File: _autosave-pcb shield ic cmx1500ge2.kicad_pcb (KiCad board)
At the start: 2 copper layers, 67.9 x 53.3 mm, 52 parts, among them J1 SMA, J2 U.FL, J3 Conn_01x01_Male, J4 Conn_01x01_Male, P1 Power, P2 Analog, P3 Digital, P4 Digital, P5 HEADER2x4, P6 HEADER-1X6, P7 Communication, Q1 BSS138, Q2 BSS138, Q3 BSS138, U1 CXM1500GE, U2 TXS0108EPW, U3 LM1117-Adj, U4 ADS1115

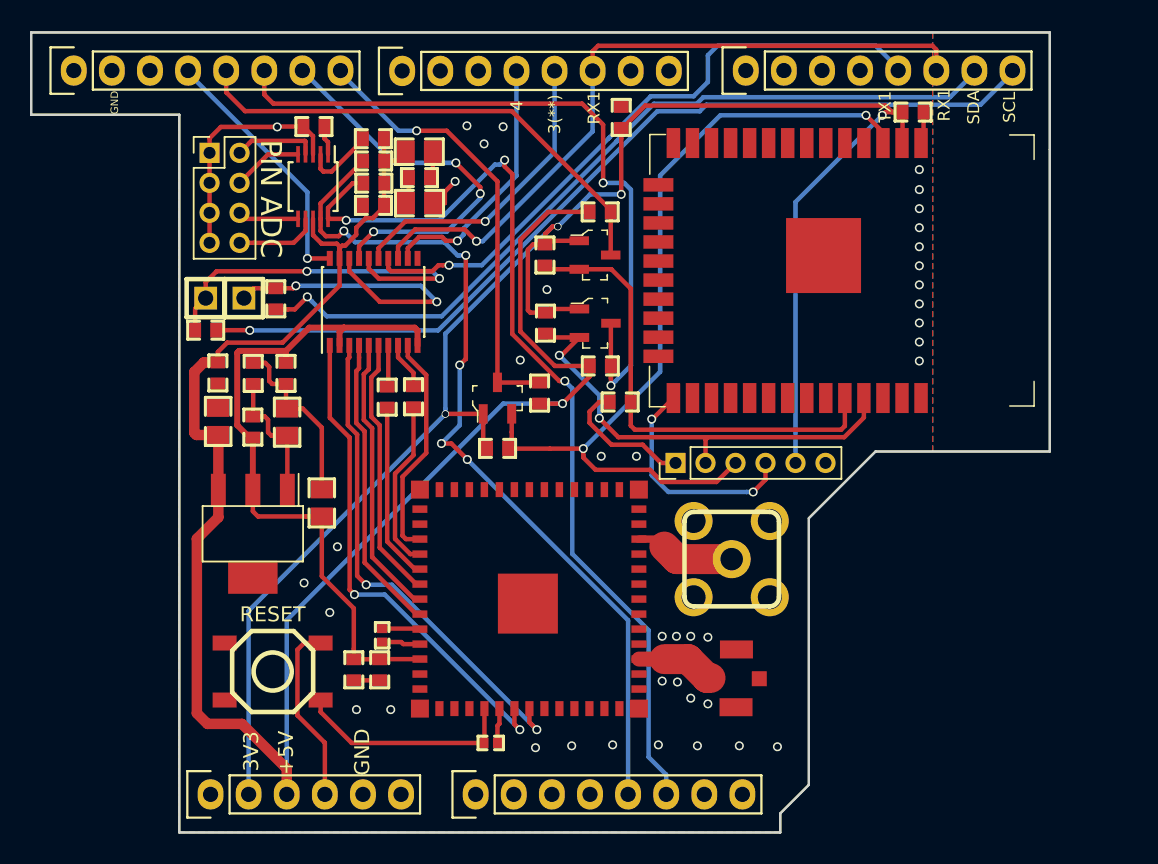
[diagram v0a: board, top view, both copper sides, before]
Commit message: initial Commit
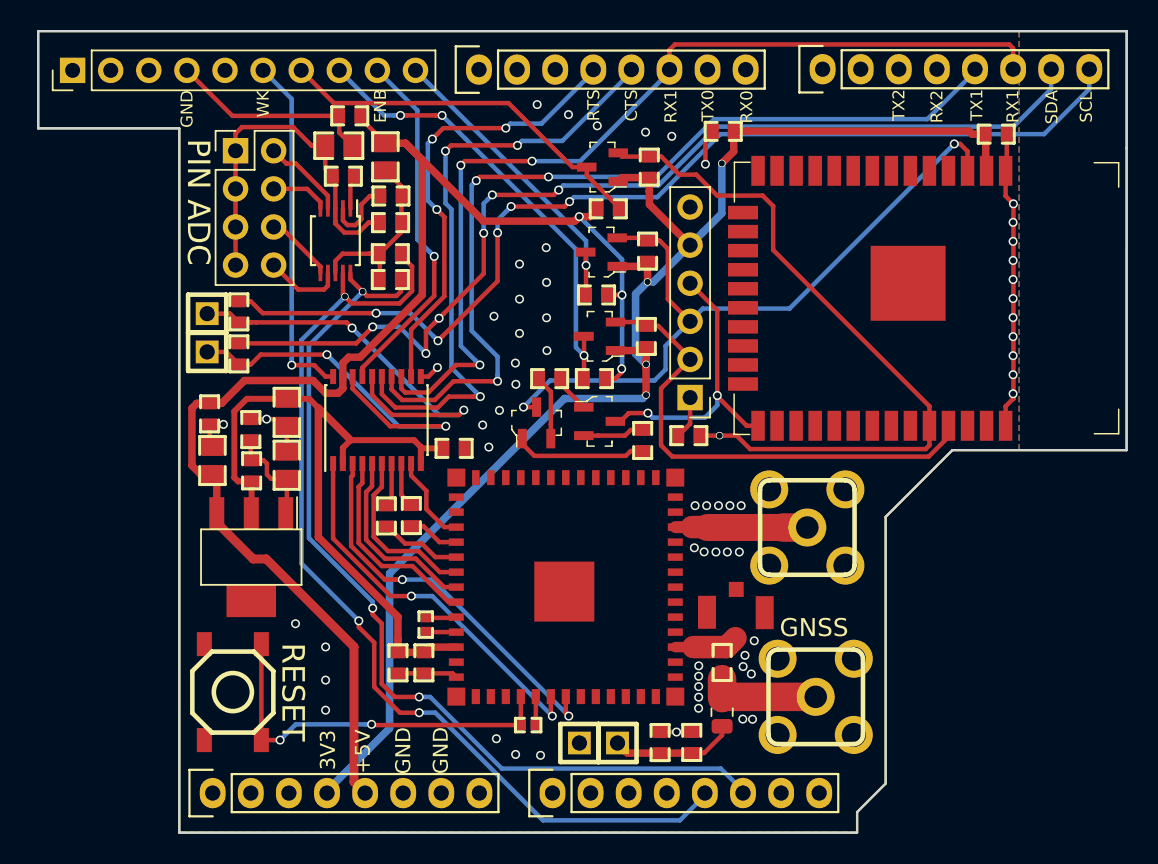
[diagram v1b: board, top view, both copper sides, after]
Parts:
- removed P3: Digital, Socket_Arduino_Uno:Socket_Strip_Arduino_1x08
- added C12: 10uF, Capasitor:C_Ceramic_SMD_0603, F.Cu at (145.2, 120.4)
- added C13: 1uF, Capasitor:C_Ceramic_SMD_0603, F.Cu at (143.1, 120.4)
- added C14: 0.1u, Capasitor:C_Ceramic_SMD_0603, F.Cu at (147.2, 115.0)
- added J5: SMA, Connectors_SMA:SMA_Male_Angled_TH, F.Cu at (153.4, 117.3)
- added J6: GND, Headers:Pin_Header_1x01_Male_10mil_Straight_TH, F.Cu at (137.7, 120.4)
- added J7: VCC, Headers:Pin_Header_1x01_Male_10mil_Straight_TH, F.Cu at (140.2, 120.4)
- added J8: Conn_01x10, Connector_PinHeader_2.54mm:PinHeader_1x10_P2.54mm_Vertical, F.Cu at (103.9, 75.6)
- added L1: 35nH, Inductor:L_0805_2012Metric, F.Cu at (147.2, 118.3)
- added Q4: S8050, digikey-footprints:SOT-23-3, F.Cu at (134.8, 99.1)
- added Q5: S8050, digikey-footprints:SOT-23-3, F.Cu at (139.0, 99.0)
- added R20: 10K, resistor:R_Chip_SMD_0603, F.Cu at (135.7, 96.1)
- added R21: 10K, resistor:R_Chip_SMD_0603, F.Cu at (141.9, 100.2)
- C5: value 10uf -> 100uf
- P1: value Power -> Analog; footprint Socket_Arduino_Uno:Socket_Strip_Arduino_1x06 -> Socket_Arduino_Uno:Socket_Strip_Arduino_1x08
- P5: footprint Connector_PinHeader_2.00mm:PinHeader_2x04_P2.00mm_Vertical -> Connector_PinHeader_2.54mm:PinHeader_2x04_P2.54mm_Vertical
- P6: footprint Connector_PinHeader_2.00mm:PinHeader_1x06_P2.00mm_Vertical -> Connector_PinHeader_2.54mm:PinHeader_1x06_P2.54mm_Vertical
- moved R10 16.5 mm to (142.2, 87.6), turned to 90 degrees
- moved C2 12.3 mm to (129.3, 100.8), turned to 180 degrees
- moved Q2 12.0 mm to (139.1, 87.7), turned to 180 degrees
- moved R9 9.09 mm to (142.3, 82.0), turned to 90 degrees
- moved R5 7.92 mm to (126.5, 105.2)
- moved R6 7.92 mm to (124.8, 105.3)
- moved U2 7.88 mm to (124.2, 98.9)
- moved R13 7.57 mm to (138.8, 90.5), turned to 0 degrees
- moved C11 6.86 mm to (147.3, 79.6), turned to 180 degrees
- moved R12 6.78 mm to (142.1, 93.3), turned to 270 degrees
- moved FB2 6.60 mm to (121.6, 80.6), turned to 180 degrees
- moved R17 6.52 mm to (125.1, 89.5), turned to 180 degrees
- moved C1 6.47 mm to (118.2, 98.4), turned to 270 degrees
- moved R18 6.28 mm to (125.1, 87.8), turned to 180 degrees
- moved C7 6.21 mm to (122.4, 78.6)
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- renumbered RESET to PB1
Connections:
- net Net-(P7-Pad3) renamed /16(Tx2)
- net Net-(P7-Pad4) renamed /17(Rx2)
- C6 pad 2: +5V -> Net-(C6-Pad2)
- FB1 pad 2: +5V -> Net-(C6-Pad2)
- P1 pad 2: +3V3 -> Net-(P1-Pad2)
- P1 pad 3: +5V -> Net-(P1-Pad3)
- P1 pad 4: GND -> +3V3
- P1 pad 5: GND -> +5V
- P1 pad 6: Net-(P1-Pad6) -> GND
- R16 pad 2: +5V -> Net-(C6-Pad2)
- R17 pad 2: +5V -> Net-(C6-Pad2)
- R18 pad 2: +5V -> Net-(C6-Pad2)
- U4 pad 8: +5V -> Net-(C6-Pad2)
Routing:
- net +3V3: track 122.8 -> 93.2 mm
- net +5V: track 123.5 -> 95.4 mm, vias 1 -> 3
- net GND: track 29.7 -> 50.4 mm, vias 38 -> 62
- net /3(**)_H: track 20.5 -> 40.5 mm, vias 1 -> 3
- net /10(**_SS)_H: track 48.8 -> 30.9 mm, vias 2 -> 3
- net /18(Tx1)_H: track 42.8 -> 59.4 mm, vias 1 -> 3
- net /19(Rx1)_H: track 47.5 -> 63.3 mm, vias 1 -> 3
- net /RX_LOW: track 32.7 -> 47.9 mm, vias 0 -> 1
- net /20(SDA)_H: track 54.4 -> 67.6 mm, vias 1 -> 6
- net /4_H: track 17.4 -> 30.1 mm, vias 1 -> 3
- net Net-(C6-Pad2): track 0.00 -> 12.3 mm
- net Net-(PB1-Pad2): track 14.8 -> 26.1 mm, vias 0 -> 2
- net /8_H: track 29.8 -> 20.6 mm
- net /RTS_IC_L: track 15.1 -> 5.95 mm
- net /RTS: track 0.00 -> 8.84 mm
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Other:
- board size 67.9 x 53.3 mm -> 72.6 x 53.4 mm
- net class power: trace_width 0.7 -> 0.5
- net class rf: trace_width 2 -> 1.9
- board text added: "CTS"
- board text added: "ENB"
- board text added: "GNSS"
- board text added: "RESET"
- board text added: "RTS"
- board text added: "RX0"
- board text added: "RX2"
- board text added: "TX0"
- board text added: "TX2"
- board text added: "WK"
- board text removed: "3(**)"
- board text removed: "4"
